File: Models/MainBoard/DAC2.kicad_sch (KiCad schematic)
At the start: 11 parts, among them U5 DAC81401

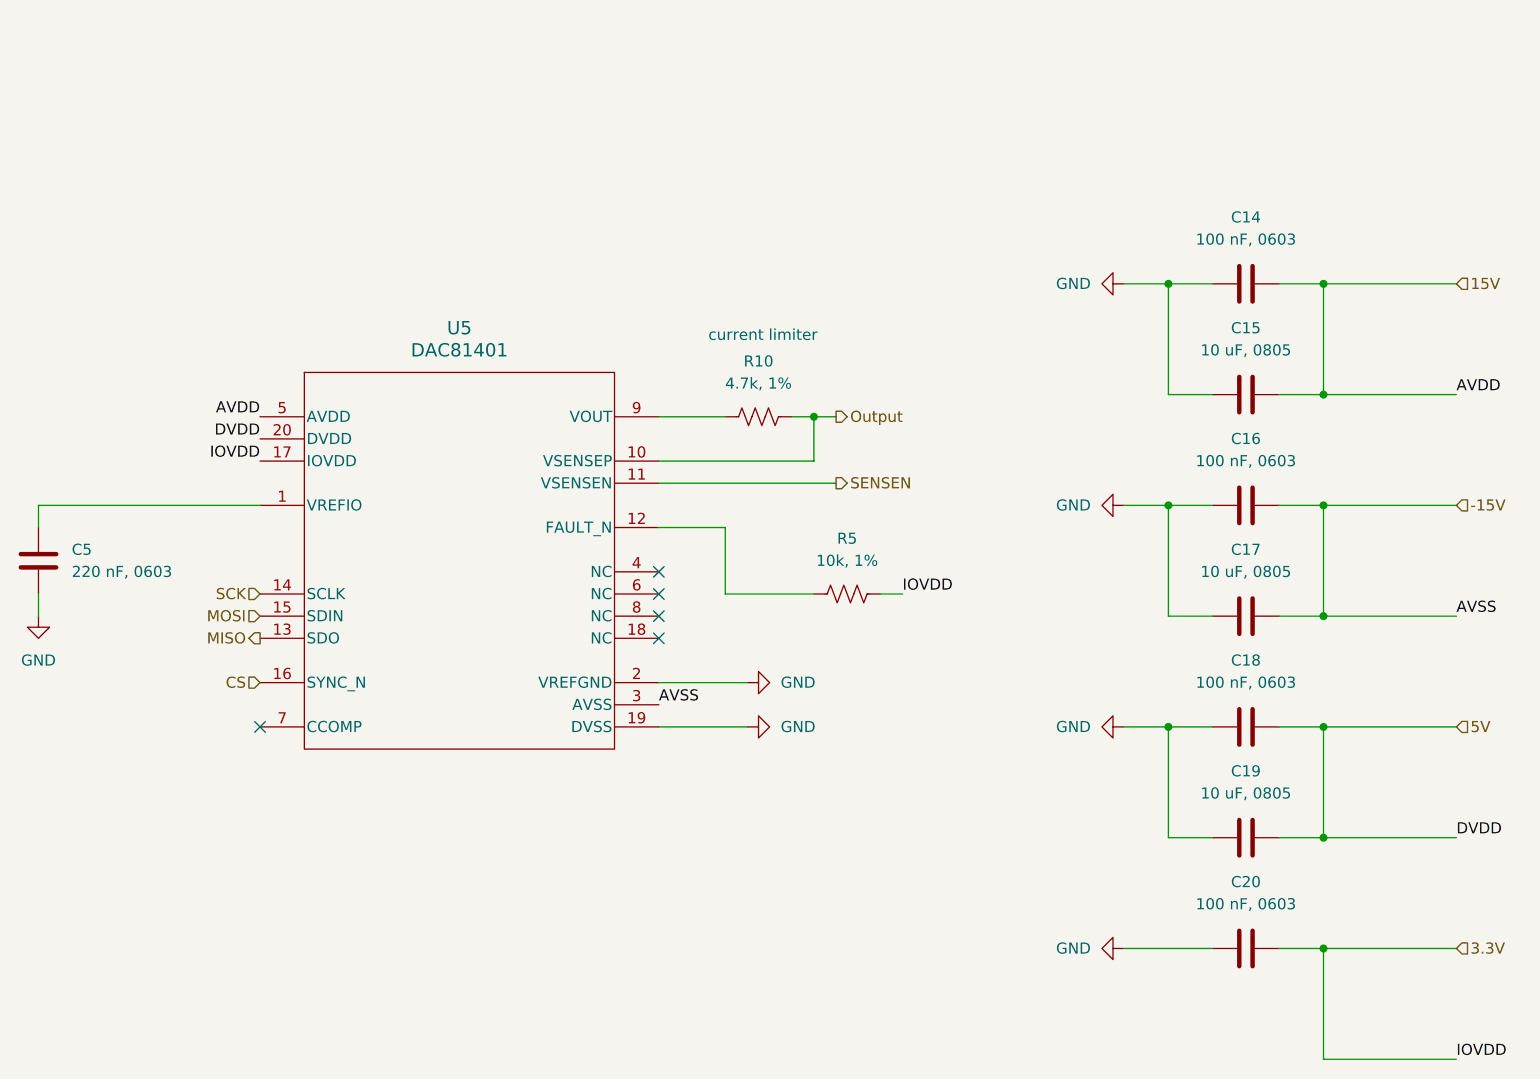
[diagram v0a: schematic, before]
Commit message: Save progress
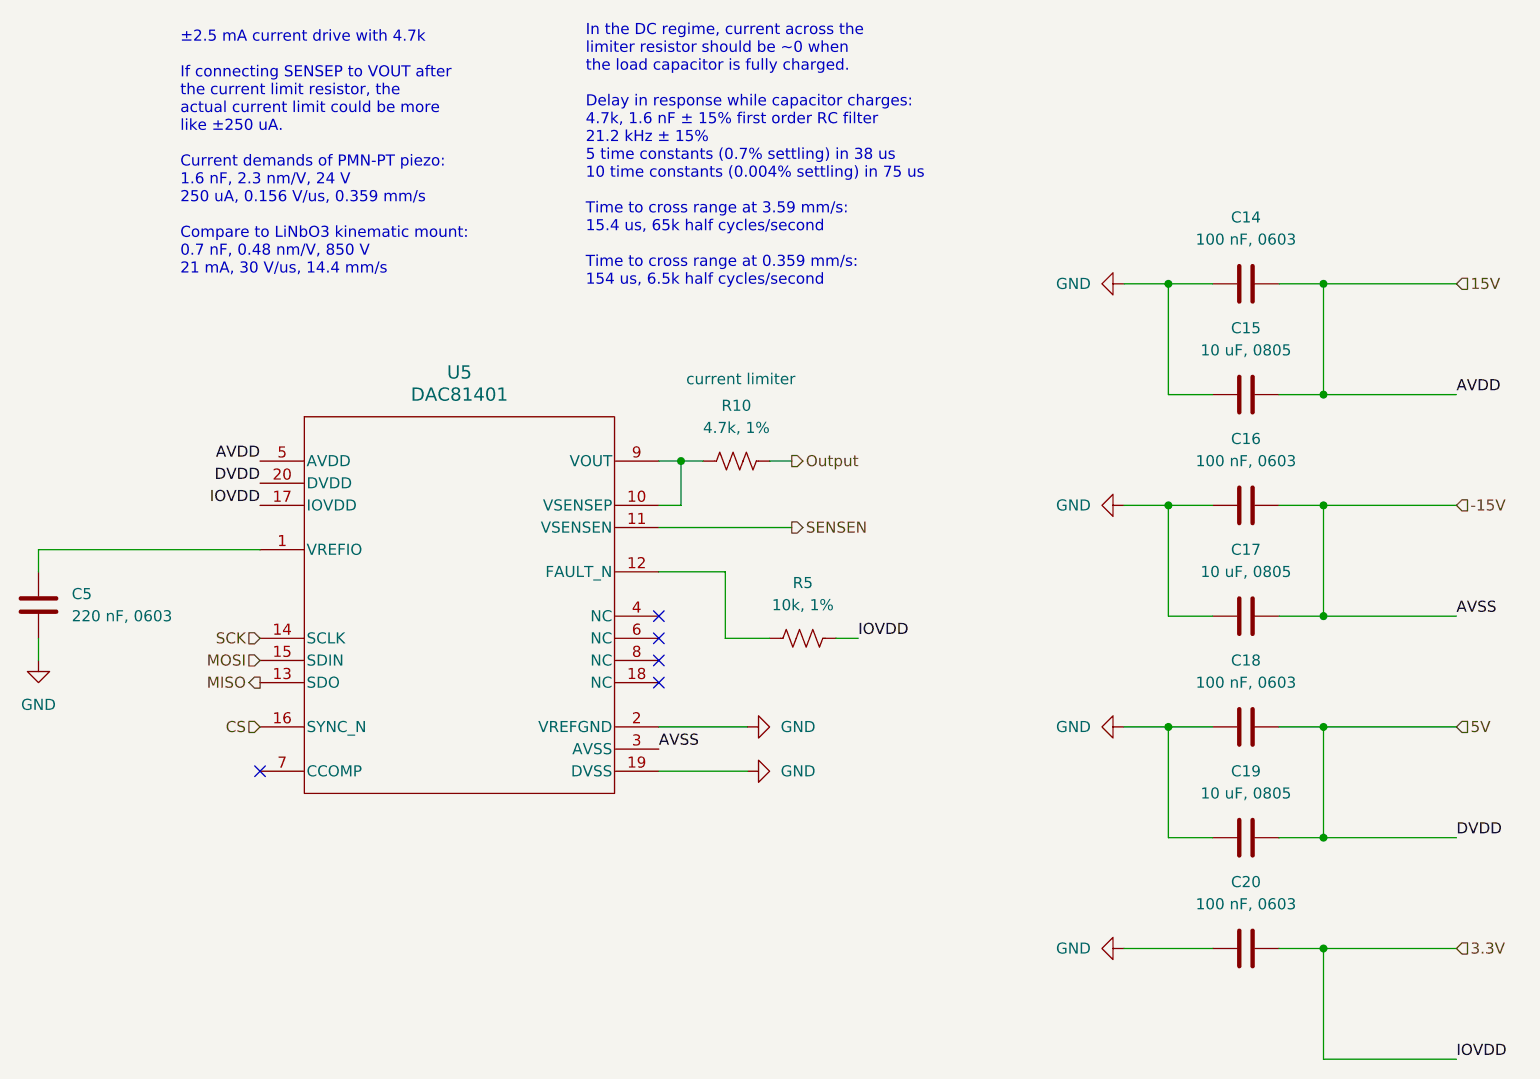
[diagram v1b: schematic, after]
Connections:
- net Output: no longer U5.10 (VSENSEP)
- net at R10.1, U5.9 (VOUT): now also U5.10 (VSENSEP)
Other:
- note added: "In the DC regime, current across the limiter resistor should be ~0 when the load capacitor is fully charged. Delay in response while capacitor charges: 4.7k, 1.6 nF ± 15% first order RC filter 21.2 kHz ± 15% 5 time constants (0.7% settling) in 38 us 10 time constants (0.004% settling) in 75 us Time to cross range at 3.59 mm/s: 15.4 us, 65k half cycles/second Time to cross range at 0.359 mm/s: 154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"
- note added: "±2.5 mA current drive with 4.7k If connecting SENSEP to VOUT after the current limit resistor, the actual current limit could be more like ±250 uA. Current demands of PMN-PT piezo: 1.6 nF, 2.3 nm/V, 24 V 250 uA, 0.156 V/us, 0.359 mm/s Compare to LiNbO3 kinematic mount: 0.7 nF, 0.48 nm/V, 850 V 21 mA, 30 V/us, 14.4 mm/s"
- moved on the sheet: C5, R10, R5, U5
